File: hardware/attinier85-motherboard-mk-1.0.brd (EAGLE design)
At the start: 22.9 x 17.8 mm, 18 parts, among them IC1 Tiny85

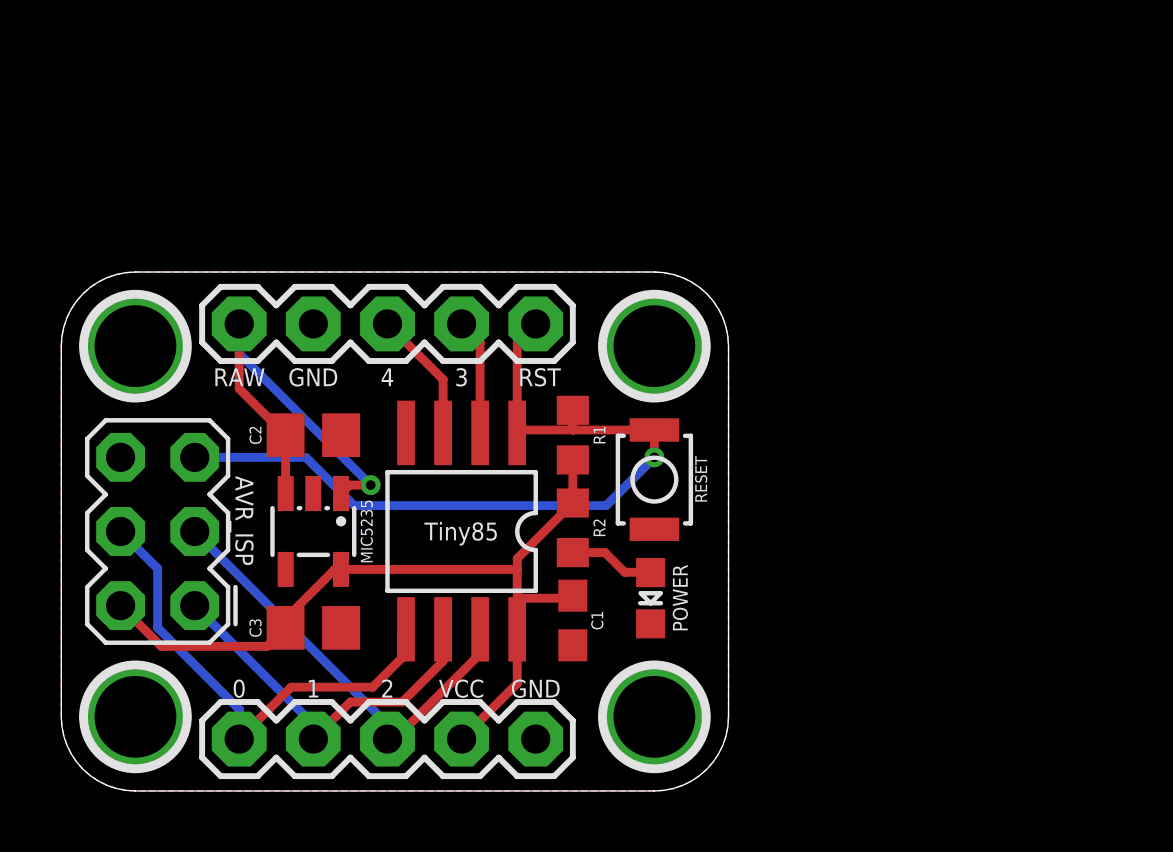
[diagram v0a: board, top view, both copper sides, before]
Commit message: cleaning up version spoo
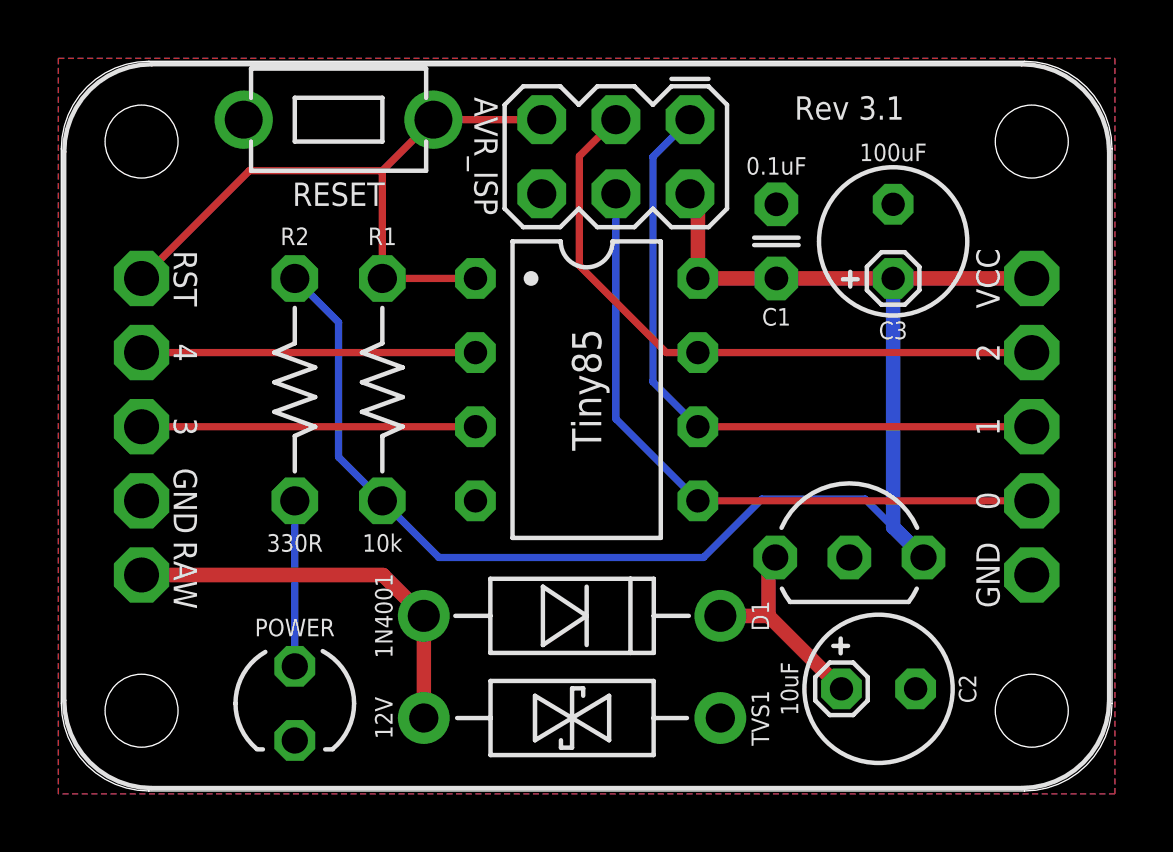
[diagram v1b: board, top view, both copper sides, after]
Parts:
- removed H1, H2, H3, H4: HOLE#2, A_butts:HOLE-#2
- removed JP1, JP2: (no value), A_butts:1X05
- removed MIC5235: V_REG_MIC5235, A_butts:SOT23-5
- added D1: 1N4001, A_butts:DIODE-10.16MM
- added IC2: LM2931, A_butts:TO-92-AMMO
- added TVS1: 12V, A_butts:DO-41-TVS
- added U1: ATTINIER85_SHIELDV2, A_butts:ATTINIER85_SHIELD_V2
- C1: value 1uF -> 0.1uF; device A_butts:C0603 -> A_butts:C025-024X044
- C2: value 1uF -> 10uF; device A_butts:C0805 -> A_butts:E2,5-5
- C3: value 10uF -> 100uF; device A_butts:C0805 -> A_butts:E2,5-5
- IC1: device A_butts:SO08-EIAJ -> A_butts:DIP08
- POWER: value LED0603 -> LED3MM-LESS; device A_butts:LED-0603 -> A_butts:LED3MM-LESSSILK
- R1, R2: device A_butts:R0603 -> A_butts:RESISTOR-AXIAL-PTH-7.62MM
- RESET: value SPST-NO-TACTB3U-1000P -> DTS-6MM; device A_butts:B3U-1000P -> A_butts:DTS-3-SMALL-PADS
- moved C3 23.9 mm to (28.5, 18.8), turned to 90 degrees
- moved C2 21.2 mm to (28.0, 3.50)
- moved AVR_ISP 20.3 mm to (19.0, 21.7), turned to 180 degrees
- moved RESET 16.4 mm to (9.50, 23.0), turned to 0 degrees
- moved C1 14.7 mm to (24.5, 18.8), turned to 90 degrees
- moved POWER 12.7 mm to (8.00, 3.00), turned to 270 degrees
- moved R2 10.6 mm to (8.00, 13.8)
- moved U$1 7.23 mm to (27.5, 12.5), turned to 0 degrees
- moved R1 6.71 mm to (11.0, 13.8), turned to 270 degrees
- moved U$2 6.58 mm to (18.0, 12.5), turned to 0 degrees
- moved IC1 6.48 mm to (18.0, 13.8), turned to 270 degrees
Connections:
- removed net D0: AVR_ISP.4, IC1.5, JP2.1
- removed net D1: AVR_ISP.1, IC1.6, JP2.2
- removed net D2: AVR_ISP.3, IC1.7, JP2.3
- new net MISO: AVR_ISP.1, IC1.6, U1.1
- new net MOSI/SDA: AVR_ISP.4, IC1.5, U1.0
- new net N$3: C2.+, D1.C, IC2.1
- new net SCK/SCL: AVR_ISP.3, IC1.7, U1.2
- net D3: now also U1.4; no longer JP1.2
- net D4: now also U1.3; no longer JP1.3
- net GND: now also C2.-, C3.-, IC2.2, POWER.K, TVS1.P$2, U1.GND@1, U1.GND@2; no longer C2.2, C3.2, JP1.4, JP2.5, MIC5235.2, MIC5235.4, POWER.C
- net N$7: now also R2.P$2; no longer R2.2
- net RAW: now also D1.A, TVS1.P$1, U1.RAW; no longer C2.1, JP1.5, MIC5235.1, MIC5235.3
- net RST: now also R1.P$1, RESET.2, U1.RST; no longer JP1.1, R1.2, RESET.0
- net VCC: now also C3.+, IC2.3, R1.P$2, R2.P$1, U1.VCC; no longer C3.1, JP2.4, MIC5235.5, R1.1, R2.1
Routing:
- net VCC: track 28.7 -> 52.8 mm
- net MOSI/SDA: track 0.00 -> 23.1 mm
- net MISO: track 0.00 -> 23.1 mm
- net SCK/SCL: track 0.00 -> 22.3 mm
- net D0: track 16.6 -> 0.00 mm
- net D2: track 15.1 -> 0.00 mm
- net D1: track 12.9 -> 0.00 mm
- net D3: track 4.00 -> 11.4 mm
- net N$3: track 0.00 -> 7.28 mm
- net D4: track 4.52 -> 11.4 mm
- net RST: track 27.5 -> 22.8 mm, vias 1 -> 0
- net N$7: track 2.95 -> 5.67 mm
- net RAW: track 15.0 -> 13.7 mm, vias 1 -> 0
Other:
- board size 22.9 x 17.8 mm -> 36 x 25 mm
- board text added: ">AUTHOR"
- board text added: ">VERSION"
- board text added: "ATTinier85"
- board text removed: "0"
- board text removed: "1"
- board text removed: "2"
- board text removed: "3"
- board text removed: "4"
- board text removed: "GND"
- board text removed: "RAW"
- board text removed: "RST"
- board text removed: "VCC"
